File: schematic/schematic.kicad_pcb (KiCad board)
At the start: 2 copper layers, 45 parts, among them J1 Conn_ARM_SWD_TagConnect_TC203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, SW1 SW_Push, U1 STM32H743VITx, U2 AMS1117, U3 TB6612FNG_C_8_EL, U4 MP1584, Y1 Crystal_GND23_Small

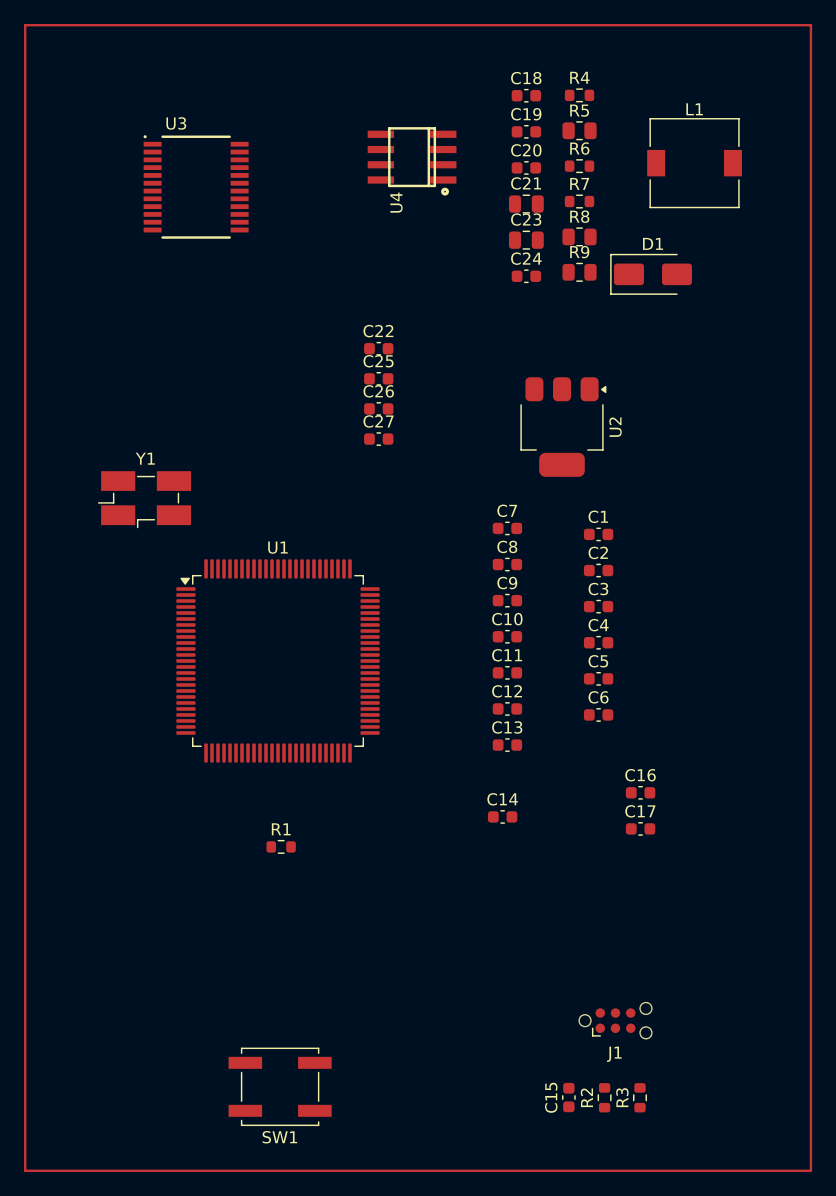
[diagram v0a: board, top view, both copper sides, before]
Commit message: xong phần nguồn
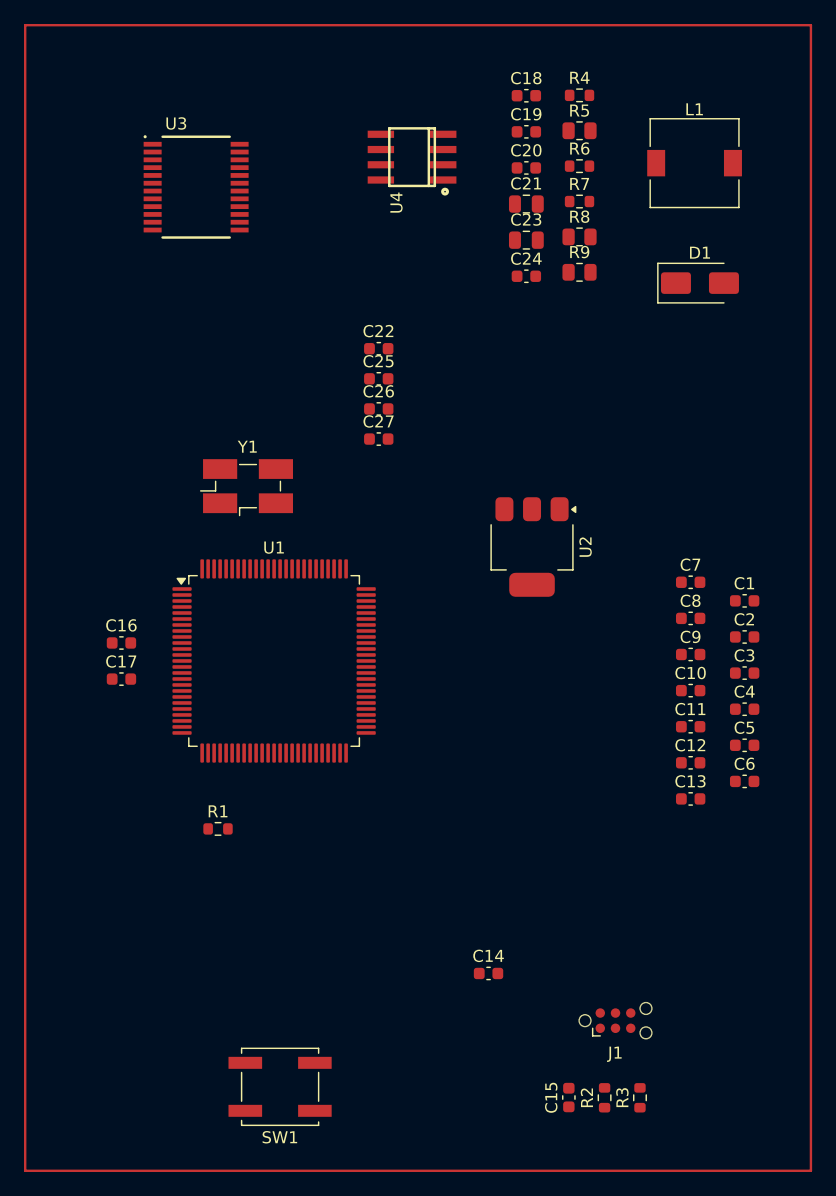
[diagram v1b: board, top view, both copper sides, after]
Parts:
- R8: value 63.4K -> 75k
- moved C16 45.0 mm to (129.3, 97.5)
- moved C17 45.0 mm to (129.3, 100.5)
- moved C11 15.9 mm to (176.7, 104.5)
- moved C8 15.9 mm to (176.7, 95.5)
- moved C10 15.9 mm to (176.7, 101.5)
- moved C12 15.9 mm to (176.7, 107.5)
- moved C13 15.9 mm to (176.7, 110.5)
- moved C7 15.9 mm to (176.7, 92.4)
- moved C9 15.9 mm to (176.7, 98.5)
- moved C2 13.4 mm to (181.2, 97.0)
- moved C3 13.4 mm to (181.2, 100.0)
- moved C5 13.4 mm to (181.2, 106.0)
- moved C6 13.4 mm to (181.2, 109.0)
- moved C1 13.4 mm to (181.2, 94.0)
- moved C4 13.4 mm to (181.2, 103.0)
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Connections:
- net 6-7.5V renamed 6.5-7.5V
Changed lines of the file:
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@@
 	(net 82 "/PH0")
 	(net 83 "+5V")
-	(net 84 "6-7.5V")
+	(net 84 "6.5-7.5V")
 	(net 85 "Net-(U4-BST)")
 	(net 86 "Net-(C21-Pad2)")
@@
 			(layers "F.Cu" "F.Paste" "F.Mask")
 			(roundrect_rratio 0.25)
-			(net 84 "6-7.5V")
+			(net 84 "6.5-7.5V")
 			(pintype "passive")
 		)
@@
 	(footprint "Capacitor_SMD:C_0603_1608Metric"
 		(layer "F.Cu")
-		(at 172.55 113)
+		(at 129.275 100.51)
 		(descr "Capacitor SMD 0603 (1608 Metric), square (rectangular) end terminal, IPC_7351 nominal, (Body size source: IPC-SM-782 page 76, https://www.pcb-3d.com/wordpress/wp-content/uploads/ipc-sm-782a_amendment_1_and_2.pdf), generated with kicad-footprint-generator")
 		(tags "capacitor")
@@
 	(footprint "Resistor_SMD:R_0603_1608Metric"
 		(layer "F.Cu")
-		(at 142.5875 114.5)
+		(at 137.325 113)
 		(descr "Resistor SMD 0603 (1608 Metric), square (rectangular) end terminal, IPC_7351 nominal, (Body size source: IPC-SM-782 page 72, https://www.pcb-3d.com/wordpress/wp-content/uploads/ipc-sm-782a_amendment_1_and_2.pdf), generated with kicad-footprint-generator")
 		(tags "resistor")
@@
 	(footprint "Capacitor_SMD:C_0603_1608Metric"
 		(layer "F.Cu")
-		(at 172.55 109.99)
+		(at 129.275 97.5)
 		(descr "Capacitor SMD 0603 (1608 Metric), square (rectangular) end terminal, IPC_7351 nominal, (Body size source: IPC-SM-782 page 76, https://www.pcb-3d.com/wordpress/wp-content/uploads/ipc-sm-782a_amendment_1_and_2.pdf), generated with kicad-footprint-generator")
 		(tags "capacitor")
@@
 	(footprint "Capacitor_SMD:C_0603_1608Metric"
 		(layer "F.Cu")
-		(at 161.45 96.98)
+		(at 176.725 101.47)
 		(descr "Capacitor SMD 0603 (1608 Metric), square (rectangular) end terminal, IPC_7351 nominal, (Body size source: IPC-SM-782 page 76, https://www.pcb-3d.com/wordpress/wp-content/uploads/ipc-sm-782a_amendment_1_and_2.pdf), generated with kicad-footprint-generator")
 		(tags "capacitor")
@@
 	(footprint "Capacitor_SMD:C_0603_1608Metric"
 		(layer "F.Cu")
-		(at 169.05 88.45)
+		(at 181.225 93.99)
 		(descr "Capacitor SMD 0603 (1608 Metric), square (rectangular) end terminal, IPC_7351 nominal, (Body size source: IPC-SM-782 page 76, https://www.pcb-3d.com/wordpress/wp-content/uploads/ipc-sm-782a_amendment_1_and_2.pdf), generated with kicad-footprint-generator")
 		(tags "capacitor")
@@
 	(footprint "Crystal:Crystal_SMD_EuroQuartz_MJ-4Pin_5.0x3.2mm_HandSoldering"
 		(layer "F.Cu")
-		(at 131.325 85.425)
+		(at 139.825 84.425)
 		(descr "SMD Crystal EuroQuartz MJ series http://cdn-reichelt.de/documents/datenblatt/B400/MJ.pdf, hand-soldering, 5.0x3.2mm^2 package")
 		(tags "SMD SMT crystal hand-soldering")
@@
 			)
 		)
-		(property "Value" "63.4K"
+		(property "Value" "75k"
 			(at 0 1.65 0)
 			(layer "F.Fab")
@@
 			(layers "F.Cu" "F.Paste" "F.Mask")
 			(roundrect_rratio 0.243902)
-			(net 84 "6-7.5V")
+			(net 84 "6.5-7.5V")
 			(pintype "passive")
 		)
@@
 	(footprint "Capacitor_SMD:C_0603_1608Metric"
 		(layer "F.Cu")
-		(at 161.45 106.01)
+		(at 176.725 110.5)
 		(descr "Capacitor SMD 0603 (1608 Metric), square (rectangular) end terminal, IPC_7351 nominal, (Body size source: IPC-SM-782 page 76, https://www.pcb-3d.com/wordpress/wp-content/uploads/ipc-sm-782a_amendment_1_and_2.pdf), generated with kicad-footprint-generator")
 		(tags "capacitor")
@@
 		)
 		(property "Value" "2.2uF"
-			(at 0 1.43 0)
+			(at -43.275 -11.06 0)
 			(layer "F.Fab")
 			(effects
@@
 	(footprint "Capacitor_SMD:C_0603_1608Metric"
 		(layer "F.Cu")
-		(at 161.45 90.96)
+		(at 176.725 95.45)
 		(descr "Capacitor SMD 0603 (1608 Metric), square (rectangular) end terminal, IPC_7351 nominal, (Body size source: IPC-SM-782 page 76, https://www.pcb-3d.com/wordpress/wp-content/uploads/ipc-sm-782a_amendment_1_and_2.pdf), generated with kicad-footprint-generator")
 		(tags "capacitor")
@@
 	(footprint "Capacitor_SMD:C_0603_1608Metric"
 		(layer "F.Cu")
-		(at 161.45 93.97)
+		(at 176.725 98.46)
 		(descr "Capacitor SMD 0603 (1608 Metric), square (rectangular) end terminal, IPC_7351 nominal, (Body size source: IPC-SM-782 page 76, https://www.pcb-3d.com/wordpress/wp-content/uploads/ipc-sm-782a_amendment_1_and_2.pdf), generated with kicad-footprint-generator")
 		(tags "capacitor")
@@
 	(footprint "Package_TO_SOT_SMD:SOT-223-3_TabPin2"
 		(layer "F.Cu")
-		(at 166 79.5 -90)
+		(at 163.5 89.5 -90)
 		(descr "module CMS SOT223 4 pins")
 		(tags "CMS SOT")
@@
 		)
 		(fp_text user "${REFERENCE}"
-			(at 0 0 360)
+			(at 0 0 0)
 			(layer "F.Fab")
 			(effects
@@
 	(footprint "Capacitor_SMD:C_0603_1608Metric"
 		(layer "F.Cu")
-		(at 161.45 99.99)
+		(at 176.725 104.48)
 		(descr "Capacitor SMD 0603 (1608 Metric), square (rectangular) end terminal, IPC_7351 nominal, (Body size source: IPC-SM-782 page 76, https://www.pcb-3d.com/wordpress/wp-content/uploads/ipc-sm-782a_amendment_1_and_2.pdf), generated with kicad-footprint-generator")
 		(tags "capacitor")
@@
 	(footprint "Capacitor_SMD:C_0603_1608Metric"
 		(layer "F.Cu")
-		(at 161.45 103)
+		(at 176.725 107.49)
 		(descr "Capacitor SMD 0603 (1608 Metric), square (rectangular) end terminal, IPC_7351 nominal, (Body size source: IPC-SM-782 page 76, https://www.pcb-3d.com/wordpress/wp-content/uploads/ipc-sm-782a_amendment_1_and_2.pdf), generated with kicad-footprint-generator")
 		(tags "capacitor")
@@
 	(footprint "Capacitor_SMD:C_0603_1608Metric"
 		(layer "F.Cu")
-		(at 169.05 97.48)
+		(at 181.225 103.02)
 		(descr "Capacitor SMD 0603 (1608 Metric), square (rectangular) end terminal, IPC_7351 nominal, (Body size source: IPC-SM-782 page 76, https://www.pcb-3d.com/wordpress/wp-content/uploads/ipc-sm-782a_amendment_1_and_2.pdf), generated with kicad-footprint-generator")
 		(tags "capacitor")
@@
 	(footprint "Diode_SMD:D_SMA"
 		(layer "F.Cu")
-		(at 173.585 66.77)
+		(at 177.5 67.5)
 		(descr "Diode SMA (DO-214AC)")
 		(tags "Diode SMA (DO-214AC)")
@@
 	(footprint "Capacitor_SMD:C_0603_1608Metric"
 		(layer "F.Cu")
-		(at 169.05 100.49)
+		(at 181.225 106.03)
 		(descr "Capacitor SMD 0603 (1608 Metric), square (rectangular) end terminal, IPC_7351 nominal, (Body size source: IPC-SM-782 page 76, https://www.pcb-3d.com/wordpress/wp-content/uploads/ipc-sm-782a_amendment_1_and_2.pdf), generated with kicad-footprint-generator")
 		(tags "capacitor")
@@
 	(footprint "Capacitor_SMD:C_0603_1608Metric"
 		(layer "F.Cu")
-		(at 161.45 87.95)
+		(at 176.725 92.44)
 		(descr "Capacitor SMD 0603 (1608 Metric), square (rectangular) end terminal, IPC_7351 nominal, (Body size source: IPC-SM-782 page 76, https://www.pcb-3d.com/wordpress/wp-content/uploads/ipc-sm-782a_amendment_1_and_2.pdf), generated with kicad-footprint-generator")
 		(tags "capacitor")
@@
 	(footprint "Capacitor_SMD:C_0603_1608Metric"
 		(layer "F.Cu")
-		(at 169.05 94.47)
+		(at 181.225 100.01)
 		(descr "Capacitor SMD 0603 (1608 Metric), square (rectangular) end terminal, IPC_7351 nominal, (Body size source: IPC-SM-782 page 76, https://www.pcb-3d.com/wordpress/wp-content/uploads/ipc-sm-782a_amendment_1_and_2.pdf), generated with kicad-footprint-generator")
 		(tags "capacitor")
@@
 			(size 0.6 2.2)
 			(layers "F.Cu" "F.Paste" "F.Mask")
-			(net 84 "6-7.5V")
+			(net 84 "6.5-7.5V")
 			(pinfunction "VIN")
 			(pintype "input")
@@
 	(footprint "Package_QFP:LQFP-100_14x14mm_P0.5mm"
 		(layer "F.Cu")
-		(at 142.325 99)
+		(at 142 99)
 		(descr "LQFP, 100 Pin (https://www.nxp.com/docs/en/package-information/SOT407-1.pdf), generated with kicad-footprint-generator ipc_gullwing_generator.py")
 		(tags "LQFP QFP")
@@
 	(footprint "Capacitor_SMD:C_0603_1608Metric"
 		(layer "F.Cu")
-		(at 169.05 103.5)
+		(at 181.225 109.04)
 		(descr "Capacitor SMD 0603 (1608 Metric), square (rectangular) end terminal, IPC_7351 nominal, (Body size source: IPC-SM-782 page 76, https://www.pcb-3d.com/wordpress/wp-content/uploads/ipc-sm-782a_amendment_1_and_2.pdf), generated with kicad-footprint-generator")
 		(tags "capacitor")
@@
 	(footprint "Capacitor_SMD:C_0603_1608Metric"
 		(layer "F.Cu")
-		(at 169.05 91.46)
+		(at 181.225 97)
 		(descr "Capacitor SMD 0603 (1608 Metric), square (rectangular) end terminal, IPC_7351 nominal, (Body size source: IPC-SM-782 page 76, https://www.pcb-3d.com/wordpress/wp-content/uploads/ipc-sm-782a_amendment_1_and_2.pdf), generated with kicad-footprint-generator")
 		(tags "capacitor")
@@
 	(footprint "Capacitor_SMD:C_0603_1608Metric"
 		(layer "F.Cu")
-		(at 161.05 112)
+		(at 159.875 125.05)
 		(descr "Capacitor SMD 0603 (1608 Metric), square (rectangular) end terminal, IPC_7351 nominal, (Body size source: IPC-SM-782 page 76, https://www.pcb-3d.com/wordpress/wp-content/uploads/ipc-sm-782a_amendment_1_and_2.pdf), generated with kicad-footprint-generator")
 		(tags "capacitor")
